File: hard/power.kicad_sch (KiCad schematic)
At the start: 0 parts

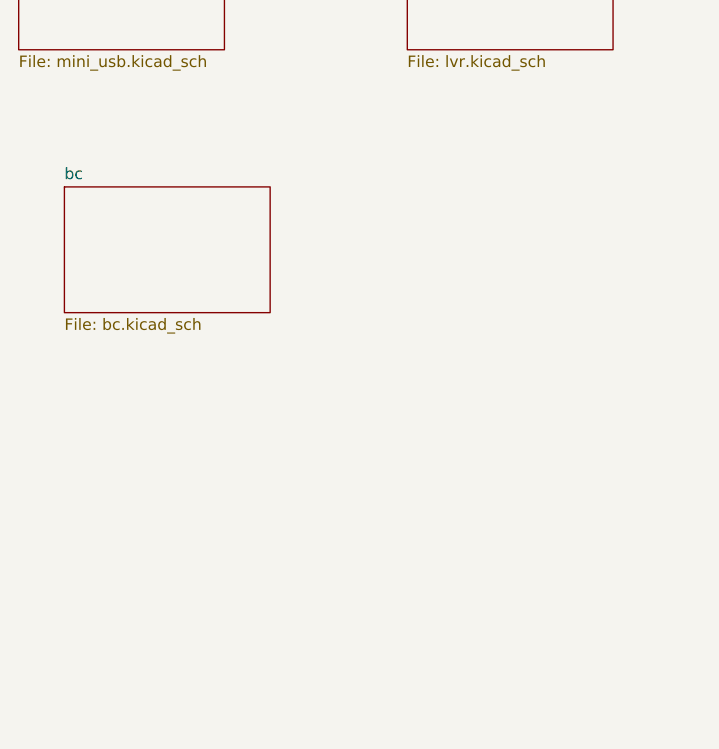
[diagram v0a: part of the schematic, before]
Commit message: edit
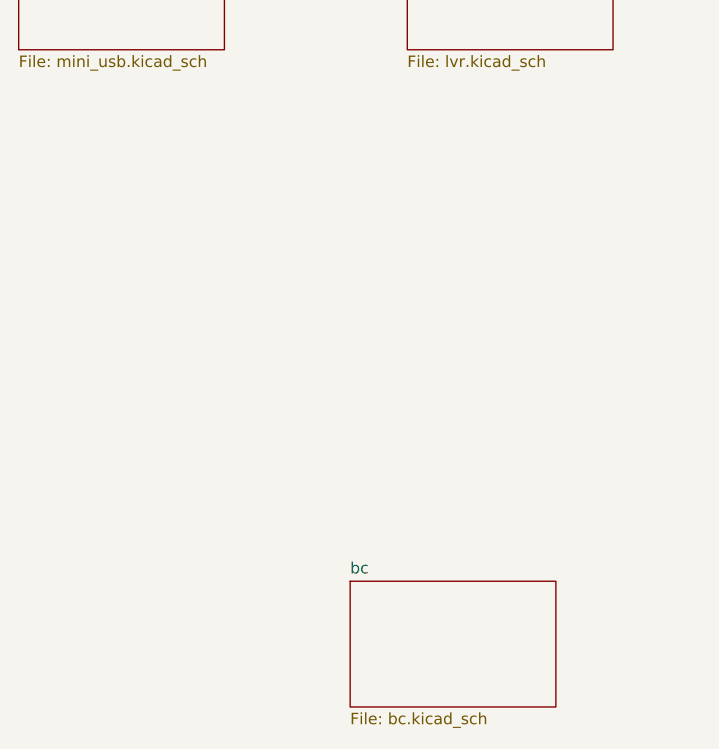
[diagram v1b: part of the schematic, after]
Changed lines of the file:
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@@
 	)
 	(sheet
-		(at 33.02 62.23)
+		(at 64.77 106.045)
 		(size 22.86 13.97)
 		(exclude_from_sim no)
@@
 		)
 		(property "Sheetname" "bc"
-			(at 33.02 61.5184 0)
+			(at 64.77 105.3334 0)
 			(effects
 				(font
@@
 		)
 		(property "Sheetfile" "bc.kicad_sch"
-			(at 33.02 76.7846 0)
+			(at 64.77 120.5996 0)
 			(effects
 				(font

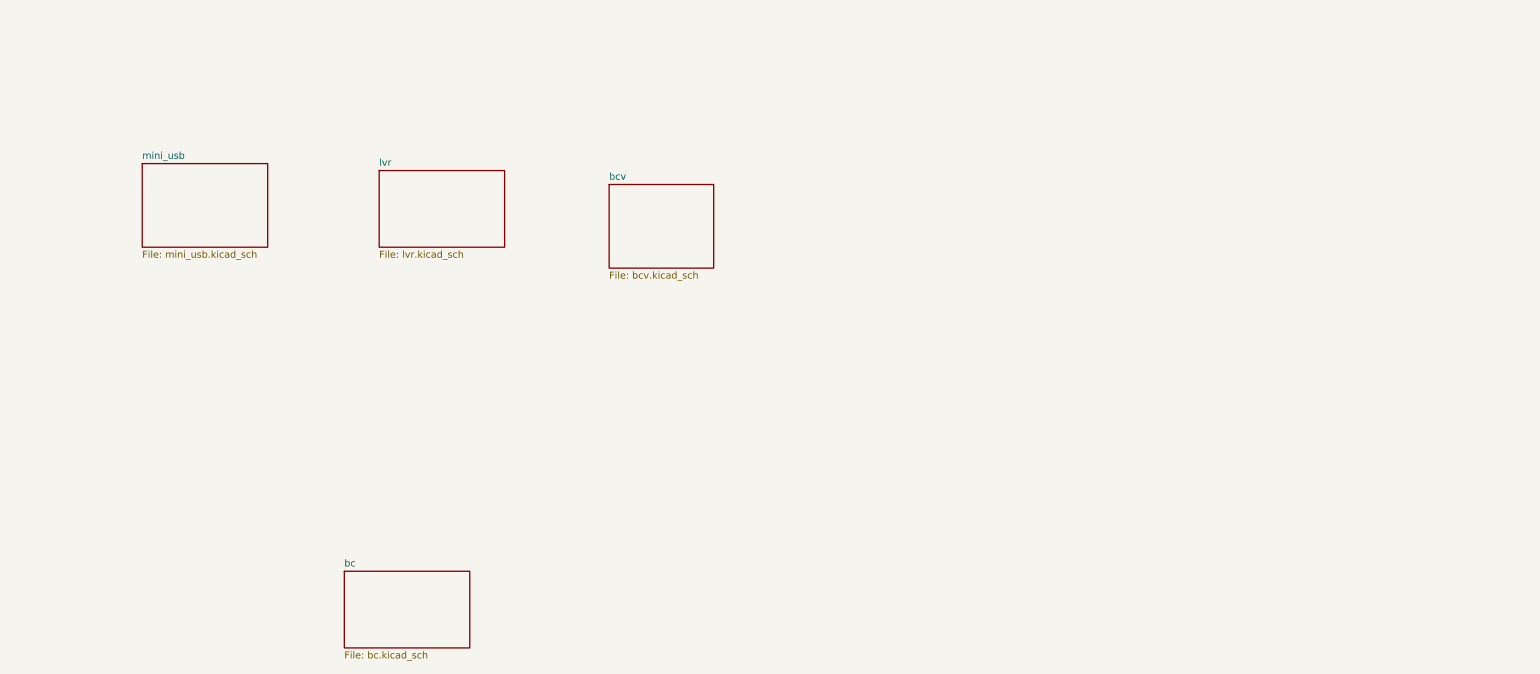
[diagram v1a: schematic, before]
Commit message: update
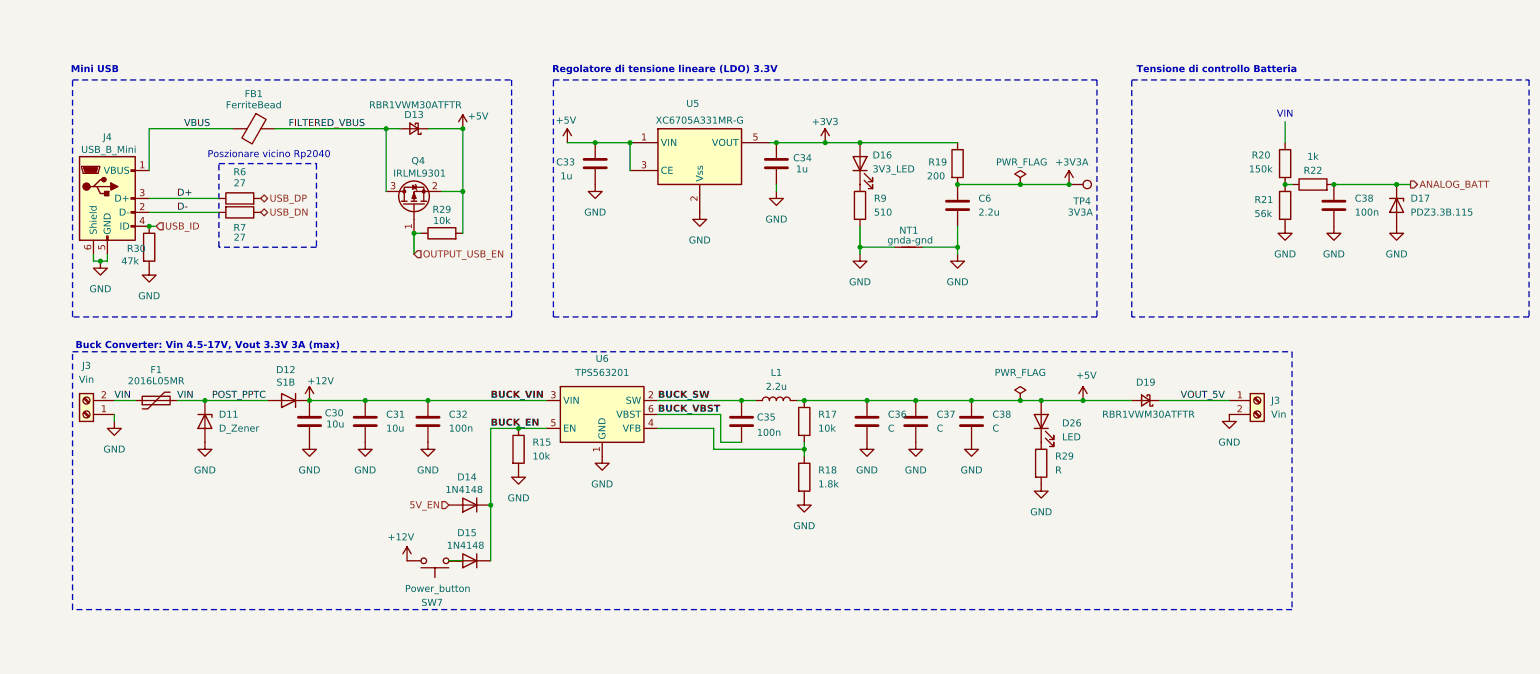
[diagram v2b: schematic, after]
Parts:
- added C30, C31: 10u, symbol Device:C
- added C32, C35, C38: 100n, symbol Device:C
- added C33, C34: 1u, symbol Device:C
- added C36, C37, C38: C, symbol Device:C
- added C6: 2.2u, symbol Device:C
- added D11: D_Zener, symbol Device:D_Zener
- added D12: S1B, symbol Device:D
- added D13, D19: RBR1VWM30ATFTR, symbol Device:D_Schottky_Small
- added D14, D15: 1N4148, symbol Device:D
- added D16: 3V3_LED, symbol Device:LED
- added D17: PDZ3.3B.115, symbol Device:D_Zener
- added D26: LED, symbol Device:LED
- added F1: 2016L05MR, symbol Device:Polyfuse
- added FB1: FerriteBead, symbol Device:FerriteBead
- added J3 (x2): Vin, symbol Connector:Screw_Terminal_01x02
- added J4: USB_B_Mini, symbol Connector:USB_B_Mini
- added L1: 2.2u, symbol Device:L
- added NT1: gnda-gnd, symbol Device:NetTie_2
- added Q4: IRLML9301, Package_TO_SOT_SMD:SOT-23, symbol Transistor_FET:IRLML9301
- added R15, R17, R29: 10k, symbol Device:R
- added R18: 1.8k, symbol Device:R
- added R19: 200, symbol Device:R
- added R20: 150k, symbol Device:R
- added R21: 56k, symbol Device:R
- added R22: 1k, symbol Device:R
- added R29: R, symbol Device:R
- added R30: 47k, symbol Device:R
- added R6, R7: 27, symbol Device:R
- added R9: 510, symbol Device:R
- added SW7: Power_button, symbol Switch:SW_Push
- added TP4: 3V3A, symbol Connector:TestPoint
- added U5: XC6705A331MR-G, Package_TO_SOT_SMD:SOT-23-5, symbol Regulator_Linear:XC6210B332MR
- added U6: TPS563201, Package_SO:SOIC-8_3.9x4.9mm_P1.27mm, symbol Regulator_Switching:XL1509-5.0
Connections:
- new net: D16.1 (K), R9.1
- new net: R20.2, R21.1, R22.1
- new net: D26.1 (K), R29.1
- new net: D15.2 (A), SW7.1
- new net: R17.2, R18.1, U6.4 (VFB)
- new net +12V: C30.1, C31.1, C32.1, D12.1 (K), SW7.2, U6.3 (VIN)
- new net +3V3: C34.1, D16.2 (A), R19.1, U5.5 (VOUT)
- new net +3V3A: C6.1, R19.2, TP4.1
- new net +5V: C33.1, C36.1, C37.1, C38.1, D13.1 (K), D19.2 (A), D26.2 (A), L1.2, Q4.2 (S), R17.1, R29.2, U5.1 (VIN), U5.3 (CE)
- new net 5V_EN: D14.2 (A)
- new net ANALOG_BATT: C38.1, D17.1 (K), R22.2
- new net BUCK_EN: D14.1 (K), D15.1 (K), R15.1, U6.5 (EN)
- new net BUCK_SW: C35.2, L1.1, U6.2 (SW)
- new net BUCK_VBST: C35.1, U6.6 (VBST)
- new net D+: J4.3 (D+), R6.1
- new net D-: J4.2 (D-), R7.2
- new net FILTERED_VBUS: D13.2 (A), FB1.1, Q4.3 (D)
- new net GND: C30.2, C31.2, C32.2, C33.2, C34.2, C36.2, C37.2, C38.2, C38.2, C6.2, D11.2 (A), D17.2 (A), J3.1 (Pin_1), J3.2 (Pin_2), J4.5 (GND), J4.6 (Shield), NT1.1, NT1.2, R15.2, R18.2, R21.2, R29.2, R30.2, R9.2, U5.2 (Vss), U6.1 (GND)
- new net OUTPUT_USB_EN: Q4.1 (G), R29.1
- new net POST_PPTC: D11.1 (K), D12.2 (A), F1.1, F1.2, J3.2 (Pin_2)
- new net USB_DN: R7.1
- new net USB_DP: R6.2
- new net USB_ID: J4.4 (ID), R30.1
- new net VBUS: FB1.2, J4.1 (VBUS)
- new net VOUT_5V: D19.1 (K), J3.1 (Pin_1)
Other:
- removed sheet bc
- removed sheet bcv
- removed sheet lvr
- removed sheet mini_usb
- note added: "Buck Converter: Vin 4.5-17V, Vout 3.3V 3A (max)"
- note added: "Mini USB"
- note added: "Poszionare vicino Rp2040"
- note added: "Regolatore di tensione lineare (LDO) 3.3V"
- note added: "Tensione di controllo Batteria"
- note added: "VIN"

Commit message: update
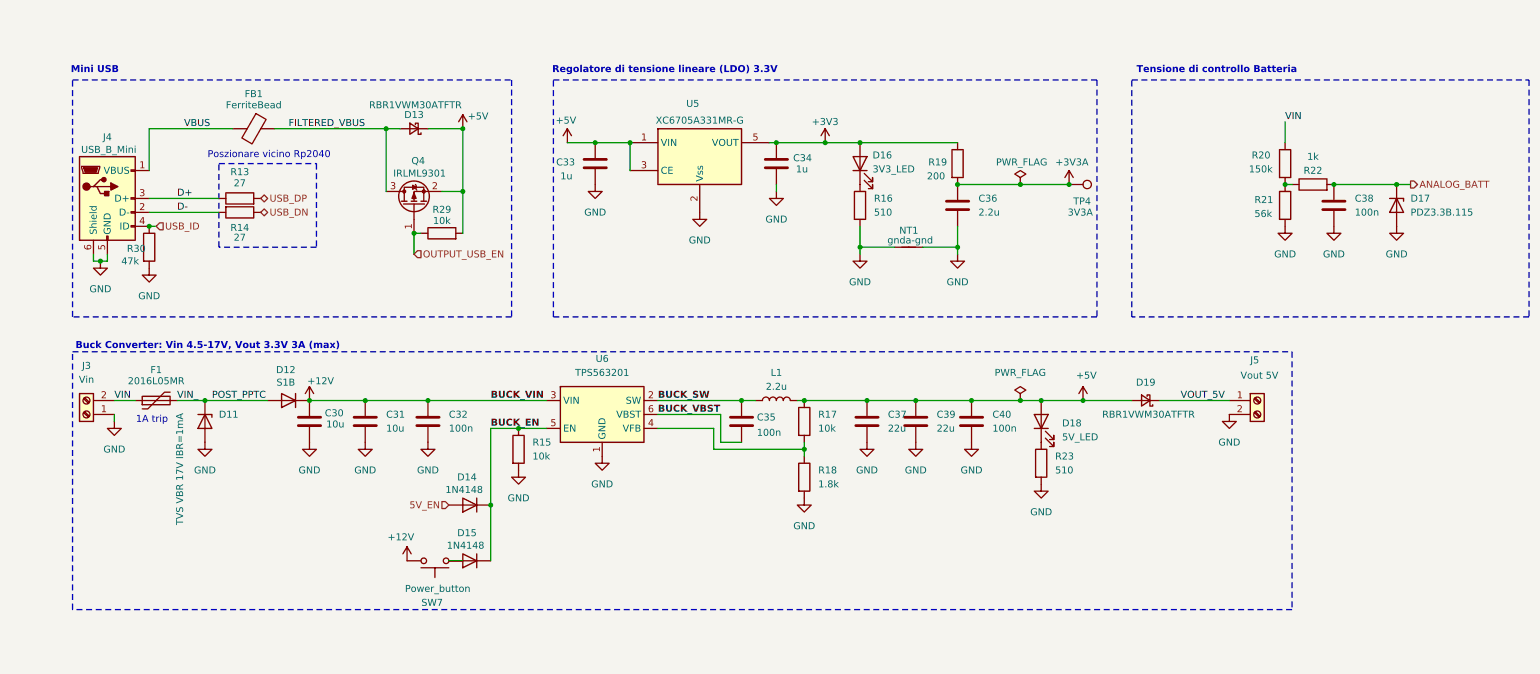
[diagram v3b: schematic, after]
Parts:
- C37: renamed from C36; value C -> 22u
- C39: renamed from C37; value C -> 22u
- C40: renamed from C38; value C -> 100n
- D11: value D_Zener -> TVS VBR 17V IBR=1mA
- D18: renamed from D26; value LED -> 5V_LED
- J5: renamed from J3; value Vin -> Vout 5V
- R23: renamed from R29; value R -> 510
- renumbered C6 to C36, R6 to R13, R7 to R14, R9 to R16
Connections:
- net POST_PPTC: no longer F1.1, J3.2 (Pin_2)
- net VIN: now reaches R20.1
- net VIN: now also F1.1, J3.2 (Pin_2)
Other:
- note added: "1A trip"
- note removed: "VIN"
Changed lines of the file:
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@@
 		)
 	)
-	(text "VIN"
+	(text "1A trip"
 		(exclude_from_sim no)
-		(at 236.22 22.86 0)
+		(at 29.718 78.486 0)
 		(effects
 			(font
@@
 		)
 	)
+	(label "VIN"
+		(at 236.22 24.13 0)
+		(effects
+			(font
+				(size 1.27 1.27)
+			)
+			(justify left bottom)
+		)
+	)
 	(label "D+"
 		(at 34.29 38.1 0)
@@
 		)
 	)
-	(label "VIN"
+	(label "VIN_"
 		(at 34.29 74.93 0)
 		(effects
@@
 		)
 		(property "Netclass" "3V3"
-			(at 159.766 22.352 0)
+			(at 160.782 22.606 0)
 			(effects
 				(font
@@
 		)
 		(property "Netclass" "TP1"
-			(at 24.384 20.828 0)
+			(at 26.924 18.542 0)
 			(effects
 				(font
@@
 		)
 		(property "Component Class" "VBUS"
-			(at 22.86 23.114 0)
+			(at 26.416 21.082 0)
 			(effects
 				(font
@@
 		(dnp no)
 		(fields_autoplaced yes)
-		(property "Reference" "C38"
+		(property "Reference" "C40"
 			(at 182.88 77.4699 0)
 			(effects
@@
 			)
 		)
-		(property "Value" "C"
+		(property "Value" "100n"
 			(at 182.88 80.0099 0)
 			(effects
@@
 			(project "PSE"
 				(path "/13844229-b559-4868-a710-53f590233cb2/ca9a428d-b29f-459a-8b79-10121d41243b"
-					(reference "C38")
+					(reference "C40")
 					(unit 1)
 				)
@@
 		(on_board yes)
 		(dnp no)
-		(property "Reference" "R7"
+		(property "Reference" "R14"
 			(at 45.72 43.434 90)
 			(effects
@@
 			(project "PSE"
 				(path "/13844229-b559-4868-a710-53f590233cb2/ca9a428d-b29f-459a-8b79-10121d41243b"
-					(reference "R7")
+					(reference "R14")
 					(unit 1)
 				)
@@
 		(dnp no)
 		(fields_autoplaced yes)
-		(property "Reference" "R29"
+		(property "Reference" "R23"
 			(at 194.31 85.0899 0)
 			(effects
@@
 			)
 		)
-		(property "Value" "R"
+		(property "Value" "510"
 			(at 194.31 87.6299 0)
 			(effects
@@
 			(project "PSE"
 				(path "/13844229-b559-4868-a710-53f590233cb2/ca9a428d-b29f-459a-8b79-10121d41243b"
-					(reference "R29")
+					(reference "R23")
 					(unit 1)
 				)
@@
 		(dnp no)
 		(fields_autoplaced yes)
-		(property "Reference" "D26"
+		(property "Reference" "D18"
 			(at 195.58 79.0574 90)
 			(effects
@@
 			)
 		)
-		(property "Value" "LED"
+		(property "Value" "5V_LED"
 			(at 195.58 81.5974 90)
 			(effects
@@
 			(project "PSE"
 				(path "/13844229-b559-4868-a710-53f590233cb2/ca9a428d-b29f-459a-8b79-10121d41243b"
-					(reference "D26")
+					(reference "D18")
 					(unit 1)
 				)
@@
 		(on_board yes)
 		(dnp no)
-		(property "Reference" "R6"
+		(property "Reference" "R13"
 			(at 45.72 33.274 90)
 			(effects
@@
 			(project "PSE"
 				(path "/13844229-b559-4868-a710-53f590233cb2/ca9a428d-b29f-459a-8b79-10121d41243b"
-					(reference "R6")
+					(reference "R13")
 					(unit 1)
 				)
@@
 		(dnp no)
 		(fields_autoplaced yes)
-		(property "Reference" "C6"
+		(property "Reference" "C36"
 			(at 180.34 38.0999 0)
 			(effects
@@
 			(project "PSE"
 				(path "/13844229-b559-4868-a710-53f590233cb2/ca9a428d-b29f-459a-8b79-10121d41243b"
-					(reference "C6")
+					(reference "C36")
 					(unit 1)
 				)
@@
 		(dnp no)
 		(fields_autoplaced yes)
-		(property "Reference" "C37"
+		(property "Reference" "C39"
 			(at 172.72 77.4699 0)
 			(effects
@@
 			)
 		)
-		(property "Value" "C"
+		(property "Value" "22u"
 			(at 172.72 80.0099 0)
 			(effects
@@
 			(project "PSE"
 				(path "/13844229-b559-4868-a710-53f590233cb2/ca9a428d-b29f-459a-8b79-10121d41243b"
-					(reference "C37")
+					(reference "C39")
 					(unit 1)
 				)
@@
 		(dnp no)
 		(fields_autoplaced yes)
-		(property "Reference" "R9"
+		(property "Reference" "R16"
 			(at 161.29 38.0999 0)
 			(effects
@@
 			(project "PSE"
 				(path "/13844229-b559-4868-a710-53f590233cb2/ca9a428d-b29f-459a-8b79-10121d41243b"
-					(reference "R9")
+					(reference "R16")
 					(unit 1)
 				)
@@
 		(on_board yes)
 		(dnp no)
-		(fields_autoplaced yes)
 		(property "Reference" "D11"
 			(at 41.91 77.4699 90)
@@
 			)
 		)
-		(property "Value" "D_Zener"
-			(at 41.91 80.0099 90)
+		(property "Value" "TVS VBR 17V IBR=1mA"
+			(at 34.798 77.216 0)
 			(effects
 				(font
@@
 		(dnp no)
 		(fields_autoplaced yes)
-		(property "Reference" "C36"
+		(property "Reference" "C37"
 			(at 163.83 77.4699 0)
 			(effects
@@
 			)
 		)
-		(property "Value" "C"
+		(property "Value" "22u"
 			(at 163.83 80.0099 0)
 			(effects
@@
 			(project "PSE"
 				(path "/13844229-b559-4868-a710-53f590233cb2/ca9a428d-b29f-459a-8b79-10121d41243b"
-					(reference "C36")
+					(reference "C37")
 					(unit 1)
 				)
@@
 		(on_board yes)
 		(dnp no)
-		(fields_autoplaced yes)
-		(property "Reference" "J3"
-			(at 233.68 74.9299 0)
+		(property "Reference" "J5"
+			(at 229.87 67.564 0)
 			(effects
 				(font
@@
 			)
 		)
-		(property "Value" "Vin"
-			(at 233.68 77.4699 0)
+		(property "Value" "Vout 5V"
+			(at 228.092 70.358 0)
 			(effects
 				(font
@@
 			(project "PSE"
 				(path "/13844229-b559-4868-a710-53f590233cb2/ca9a428d-b29f-459a-8b79-10121d41243b"
-					(reference "J3")
+					(reference "J5")
 					(unit 1)
 				)
